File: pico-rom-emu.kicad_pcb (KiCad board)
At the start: 2 copper layers, 100 x 100 mm, 37 parts, among them J1 HDR_28C256, J2 HDR_UART, J4 HDR_SWD, Q1 MMBT2222A, SW1 SW_Push, U1 74HCT574D, U2 74HCT574D, U3 74HCT574D, U4 74HCT08, U5 RaspberryPi_Pico2, U6 AS7C256C

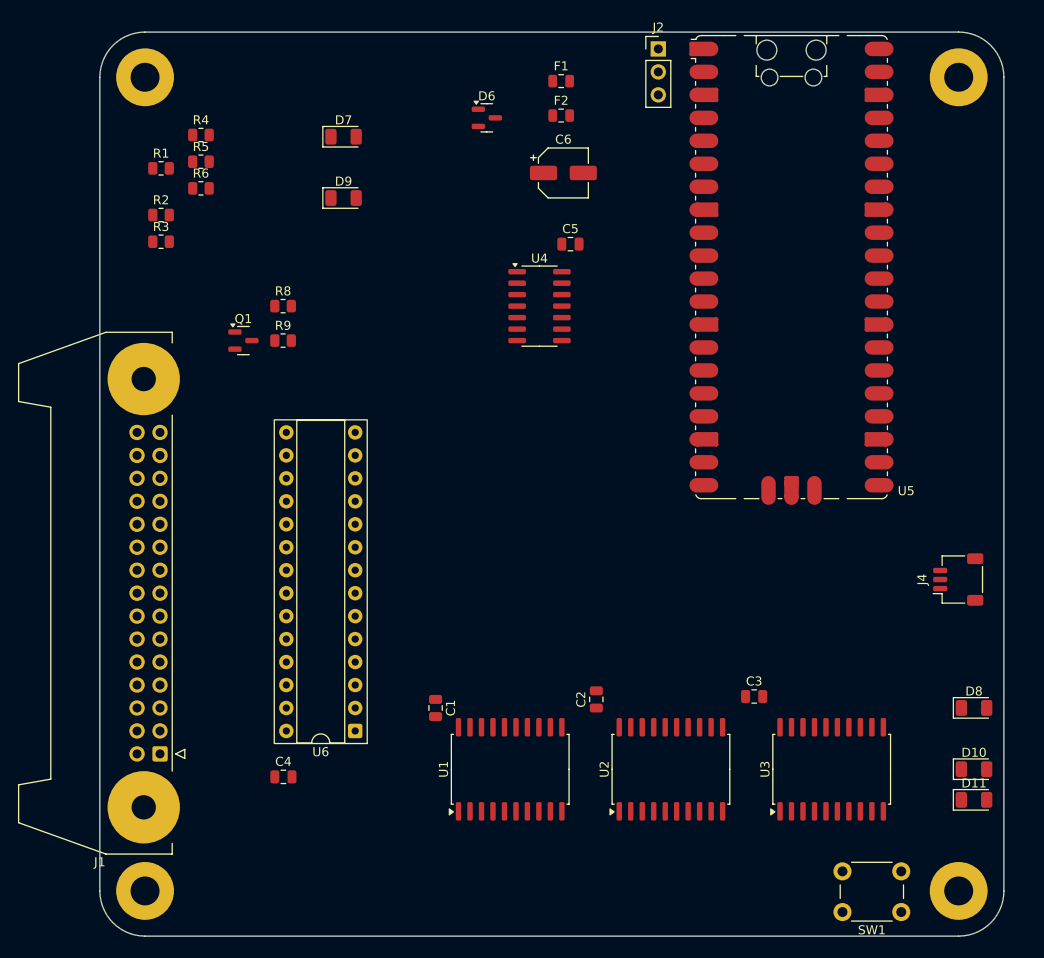
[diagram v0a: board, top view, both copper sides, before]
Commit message: pre rev1 order
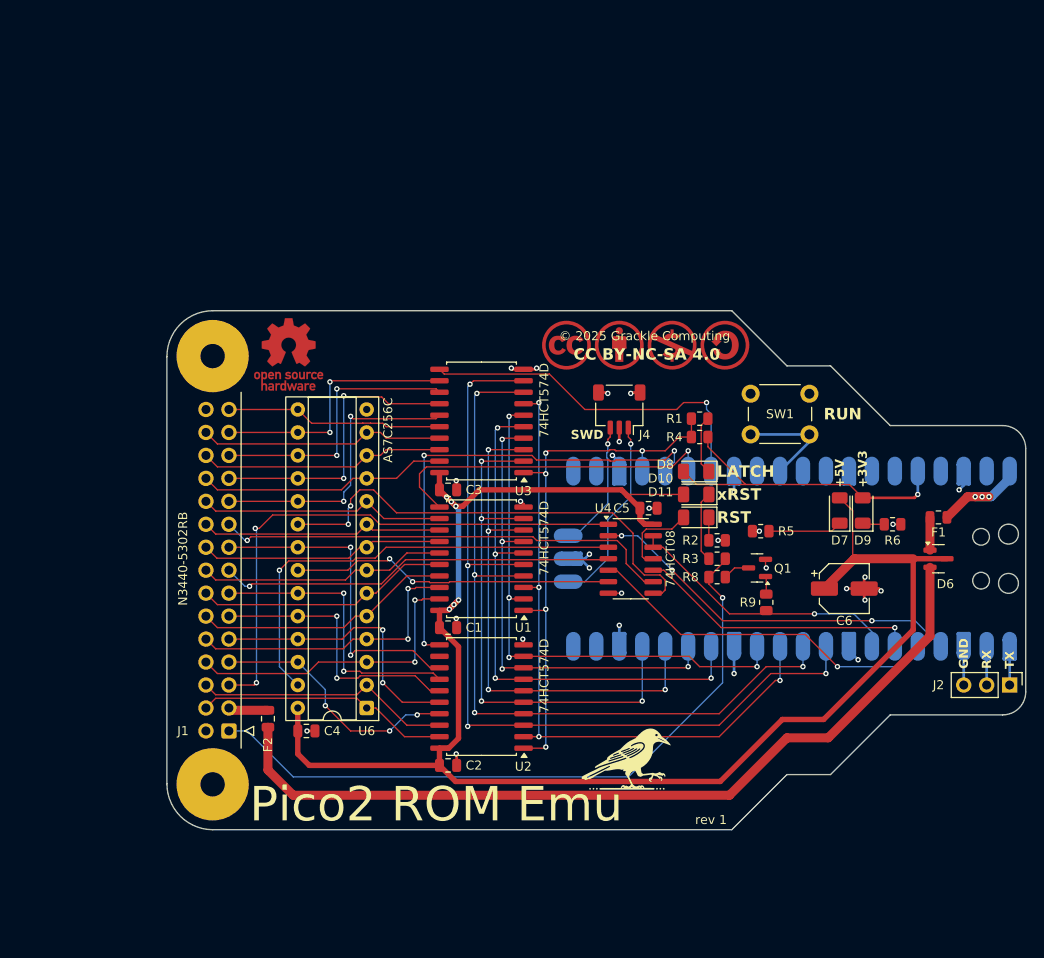
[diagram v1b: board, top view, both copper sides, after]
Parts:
- removed H1, H2, H3, H4: M3, MountingHole:MountingHole_3.2mm_M3_Pad
- added G1: LOGO, CustomSymbols:GrackleLogo12mm, F.Cu at (156.0, 127.5)
- added G3: LOGO, CustomSymbols:PCBWayLogo15x4mm, B.Cu at (139.2, 81.0)
- added REF**: OSHW-Logo_7.5x8mm_Copper, Symbol:OSHW-Logo_7.5x8mm_Copper, F.Cu at (118.4, 82.8)
- added REF**: Symbol_CC-Attribution_CopperTop_Small, Symbol:Symbol_CC-Attribution_CopperTop_Small, F.Cu at (154.9, 81.8)
- added REF**: Symbol_CC-Noncommercial_CopperTop_Small, Symbol:Symbol_CC-Noncommercial_CopperTop_Small, F.Cu at (160.8, 81.8)
- added REF**: Symbol_CreativeCommons_CopperTop_Type2_Small, Symbol:Symbol_CreativeCommons_CopperTop_Type2_Small, F.Cu at (149.1, 81.8)
- added REF**: Symbol_CC-ShareAlike_CopperTop_Small, Symbol:Symbol_CC-ShareAlike_CopperTop_Small, F.Cu at (166.6, 81.8)
- added REF**: KiCad-Logo2_8mm_SilkScreen, Symbol:KiCad-Logo2_8mm_SilkScreen, B.Cu at (158.0, 84.3)
- J1: value HDR_28C256 -> N3440-5302RB
- U5: moved to B.Cu
- moved R6 85.0 mm to (185.2, 101.6)
- moved J2 80.4 mm to (198.1, 119.4), turned to -90 degrees
- moved R5 74.2 mm to (170.6, 102.4), turned to 180 degrees
- moved F2 74.2 mm to (116.1, 123.1), turned to 90 degrees
- moved R2 71.3 mm to (165.8, 103.4)
- moved R3 70.8 mm to (165.8, 105.4)
- moved D6 69.8 mm to (190.2, 105.4)
- moved D7 68.7 mm to (179.3, 100.1), turned to 90 degrees
- moved D9 67.0 mm to (181.9, 100.1), turned to 90 degrees
- moved R1 65.7 mm to (163.8, 89.9), turned to 180 degrees
- moved R4 64.5 mm to (163.8, 91.9), turned to 180 degrees
- moved F1 63.8 mm to (190.2, 100.8), turned to 180 degrees
- moved Q1 62.1 mm to (170.2, 106.4), turned to 180 degrees
- moved R9 60.8 mm to (171.2, 110.2), turned to 90 degrees
- moved R8 56.6 mm to (165.8, 107.4), turned to 180 degrees
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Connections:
- U5 pad 10: XDA1 -> XDA5
- U5 pad 11: XDA2 -> XDA6
- U5 pad 12: XDA3 -> XDA7
- U5 pad 14: XDA4 -> XDA3
- U5 pad 15: XDA5 -> XDA2
- U5 pad 16: XDA6 -> XDA1
- U5 pad 17: XDA7 -> XDA0
- U5 pad 25: /LADL -> /LADH
- U5 pad 26: /LADH -> /LADL
- U5 pad 9: XDA0 -> XDA4
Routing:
- net +5V: track 0.00 -> 183.4 mm, vias 0 -> 6
- net XDA4: track 0.00 -> 95.3 mm, vias 0 -> 4
- net /f_x5v: track 0.00 -> 94.0 mm
- net XDA5: track 0.00 -> 86.9 mm, vias 0 -> 4
- net /X~{RST}: track 0.00 -> 75.9 mm, vias 0 -> 1
- net XDA6: track 0.00 -> 75.1 mm, vias 0 -> 4
- net XDA3: track 0.00 -> 61.4 mm, vias 0 -> 4
- net /L~{OE}: track 0.00 -> 61.3 mm, vias 0 -> 5
- net /X~{WE}: track 0.00 -> 60.4 mm, vias 0 -> 2
- net XDA7: track 0.00 -> 60.2 mm, vias 0 -> 4
- net XDA0: track 0.00 -> 59.8 mm, vias 0 -> 4
- net XDA1: track 0.00 -> 58.8 mm, vias 0 -> 4
- net /LADH: track 0.00 -> 53.7 mm, vias 0 -> 3
- net XDA2: track 0.00 -> 53.1 mm, vias 0 -> 4
- net /~{CS}: track 0.00 -> 52.4 mm, vias 0 -> 2
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- added copper zone on In1.Cu, net GND
- added copper zone on In2.Cu, net GND
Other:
- board size 100 x 100 mm -> 95 x 57.4 mm
- copper layers 2 -> 4
- board text added: "+3V3"
- board text added: "+5V"
- board text added: "1"
- board text added: "14"
- board text added: "15"
- board text added: "28"
- board text added: "74HCT08"
- board text added: "74HCT574D"
- board text added: "AS7C256C"
- board text added: "CC BY-NC-SA 4.0"
- board text added: "GND"
- board text added: "LATCH"
- board text added: "PCB Fabrication By"
- board text added: "Pico2 ROM Emu"
- board text added: "RST"
- board text added: "RUN"
- board text added: "RX"
- board text added: "SWD"
- board text added: "TX"
- board text added: "WayWayWay"
- board text added: "rev 1"
- board text added: "xRST"
- board text added: "© 2025 Grackle Computing"
